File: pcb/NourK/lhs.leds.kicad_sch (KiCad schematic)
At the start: 43 parts

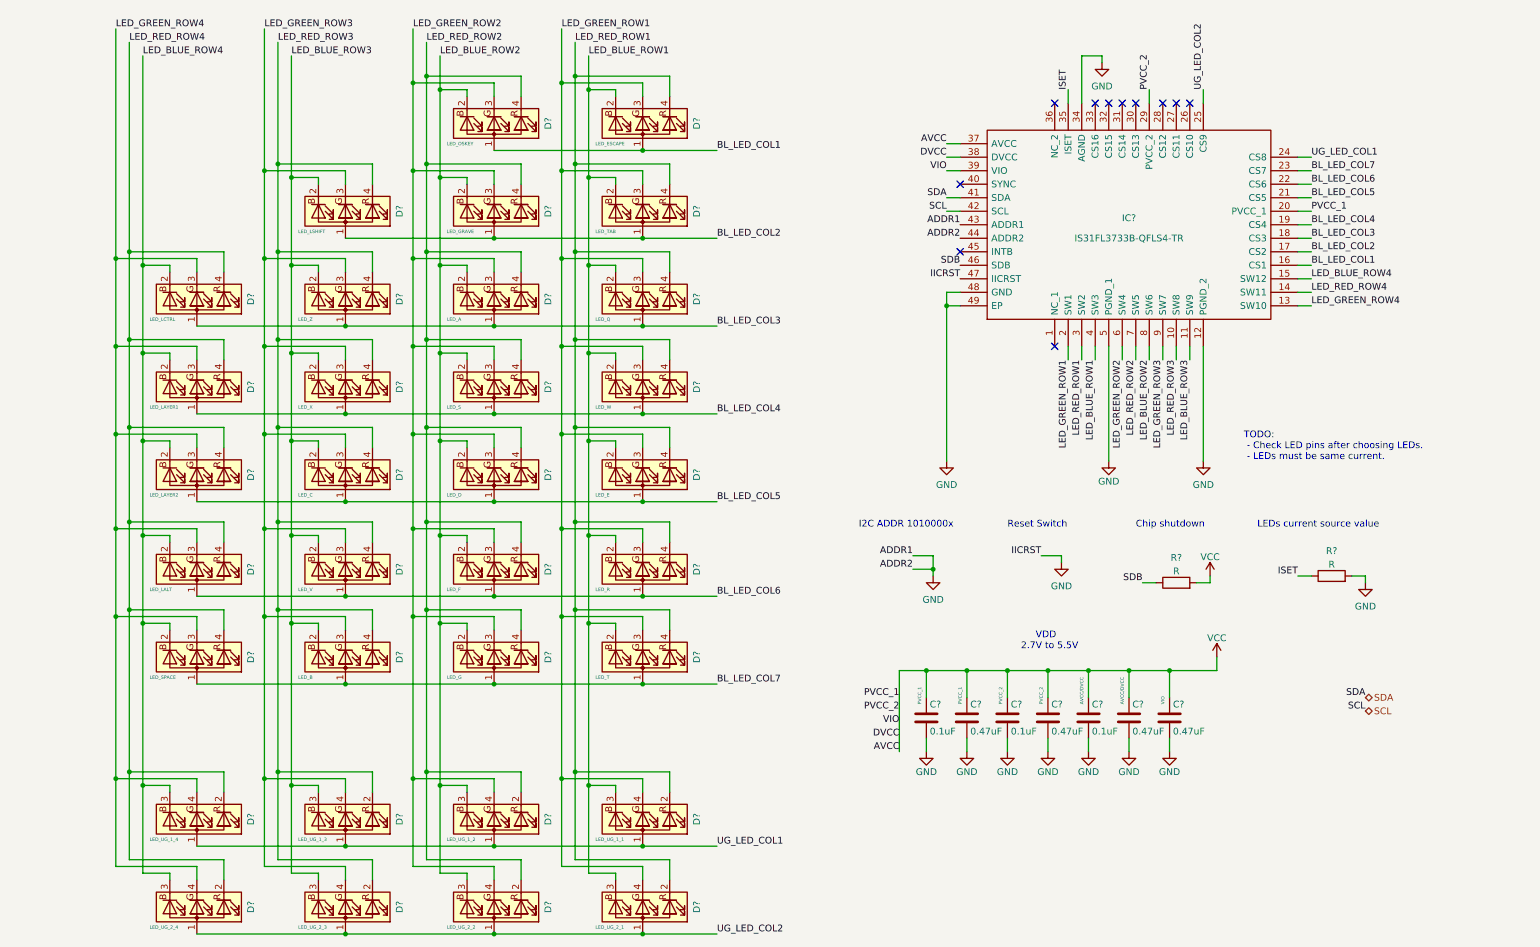
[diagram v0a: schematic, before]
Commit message: Draft LHS tracks
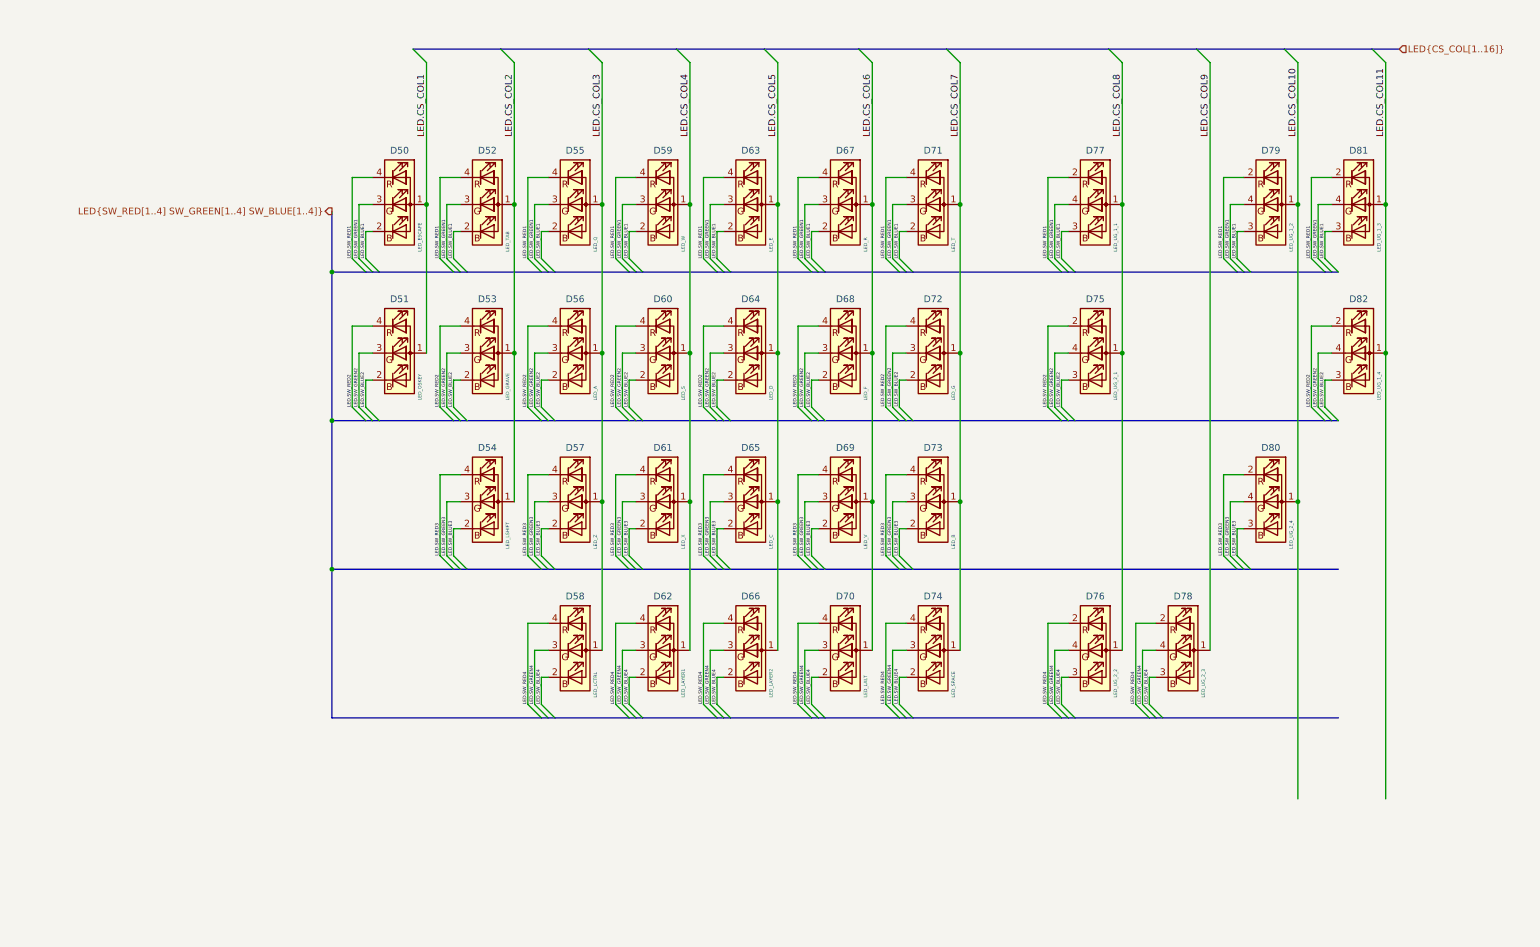
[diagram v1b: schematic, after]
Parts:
- removed C? (x3): 0.1uF, Capacitor_SMD:C_0805_2012Metric, symbol Device:C
- removed C? (x4): 0.47uF, Capacitor_SMD:C_0805_2012Metric, symbol Device:C
- removed IC?: IS31FL3733B-QFLS4-TR, Nour_KB:QFN40P600X600X80-49N-D, symbol Nour_KB:IS31FL3733B-QFLS4-TR
- removed R? (x2): R, Resistor_SMD:R_0805_2012Metric, symbol Device:R
- gave numbers to parts that had none: 33
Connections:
- net BL_LED_COL1 renamed LED.CS_COL1
- net BL_LED_COL2 renamed LED.CS_COL2
- net BL_LED_COL3 renamed LED.CS_COL3
- net BL_LED_COL4 renamed LED.CS_COL4
- net BL_LED_COL5 renamed LED.CS_COL5
- net BL_LED_COL6 renamed LED.CS_COL6
- net BL_LED_COL7 renamed LED.CS_COL7
- net LED_BLUE_ROW1 renamed LED.SW_BLUE1
- net LED.SW_BLUE1: now also D79.3 (BK), D81.3 (BK); no longer D75.3 (BK)
- net LED_BLUE_ROW2 renamed LED.SW_BLUE2
- net LED.SW_BLUE2: now also D75.3 (BK), D82.3 (BK); no longer D76.3 (BK), D79.3 (BK)
- net LED_BLUE_ROW3 renamed LED.SW_BLUE3
- net LED.SW_BLUE3: now also D80.3 (BK); no longer D78.3 (BK), D81.3 (BK)
- net LED_BLUE_ROW4 renamed LED.SW_BLUE4
- net LED.SW_BLUE4: now also D76.3 (BK), D78.3 (BK); no longer D80.3 (BK), D82.3 (BK)
- net LED_GREEN_ROW1 renamed LED.SW_GREEN1
- net LED.SW_GREEN1: now also D79.4 (GK), D81.4 (GK); no longer D75.4 (GK)
- net LED_GREEN_ROW2 renamed LED.SW_GREEN2
- net LED.SW_GREEN2: now also D75.4 (GK), D82.4 (GK); no longer D76.4 (GK), D79.4 (GK)
- net LED_GREEN_ROW3 renamed LED.SW_GREEN3
- net LED.SW_GREEN3: now also D80.4 (GK); no longer D78.4 (GK), D81.4 (GK)
- net LED_GREEN_ROW4 renamed LED.SW_GREEN4
- net LED.SW_GREEN4: now also D76.4 (GK), D78.4 (GK); no longer D80.4 (GK), D82.4 (GK)
- net LED_RED_ROW1 renamed LED.SW_RED1
- net LED.SW_RED1: now also D79.2 (RK), D81.2 (RK); no longer D75.2 (RK)
- net LED_RED_ROW2 renamed LED.SW_RED2
- net LED.SW_RED2: now also D75.2 (RK), D82.2 (RK); no longer D76.2 (RK), D79.2 (RK)
- net LED_RED_ROW3 renamed LED.SW_RED3
- net LED.SW_RED3: now also D80.2 (RK); no longer D78.2 (RK), D81.2 (RK)
- net LED_RED_ROW4 renamed LED.SW_RED4
- net LED.SW_RED4: now also D76.2 (RK), D78.2 (RK); no longer D80.2 (RK), D82.2 (RK)
- net UG_LED_COL1 renamed LED.CS_COL11
- net LED.CS_COL11: no longer D77.1 (A), D79.1 (A)
- net UG_LED_COL2 renamed LED.CS_COL8
- net LED.CS_COL8: now also D77.1 (A); no longer D78.1 (A), D80.1 (A)
- new net LED.CS_COL10: D79.1 (A), D80.1 (A)
- new net LED.CS_COL9: D78.1 (A)
- no-connect marks 11 -> 0
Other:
- note removed: "Chip shutdown"
- note removed: "I2C ADDR 1010000x"
- note removed: "LEDs current source value"
- note removed: "Reset Switch"
- note removed: "TODO: - Check LED pins after choosing LEDs. - LEDs must be same current."
- note removed: "VDD 2.7V to 5.5V"
- moved on the sheet: D50, D51, D52, D53, D54, D55, D56, D57, D58, D59, D60, D61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
